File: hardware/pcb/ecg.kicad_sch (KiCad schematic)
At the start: 0 parts

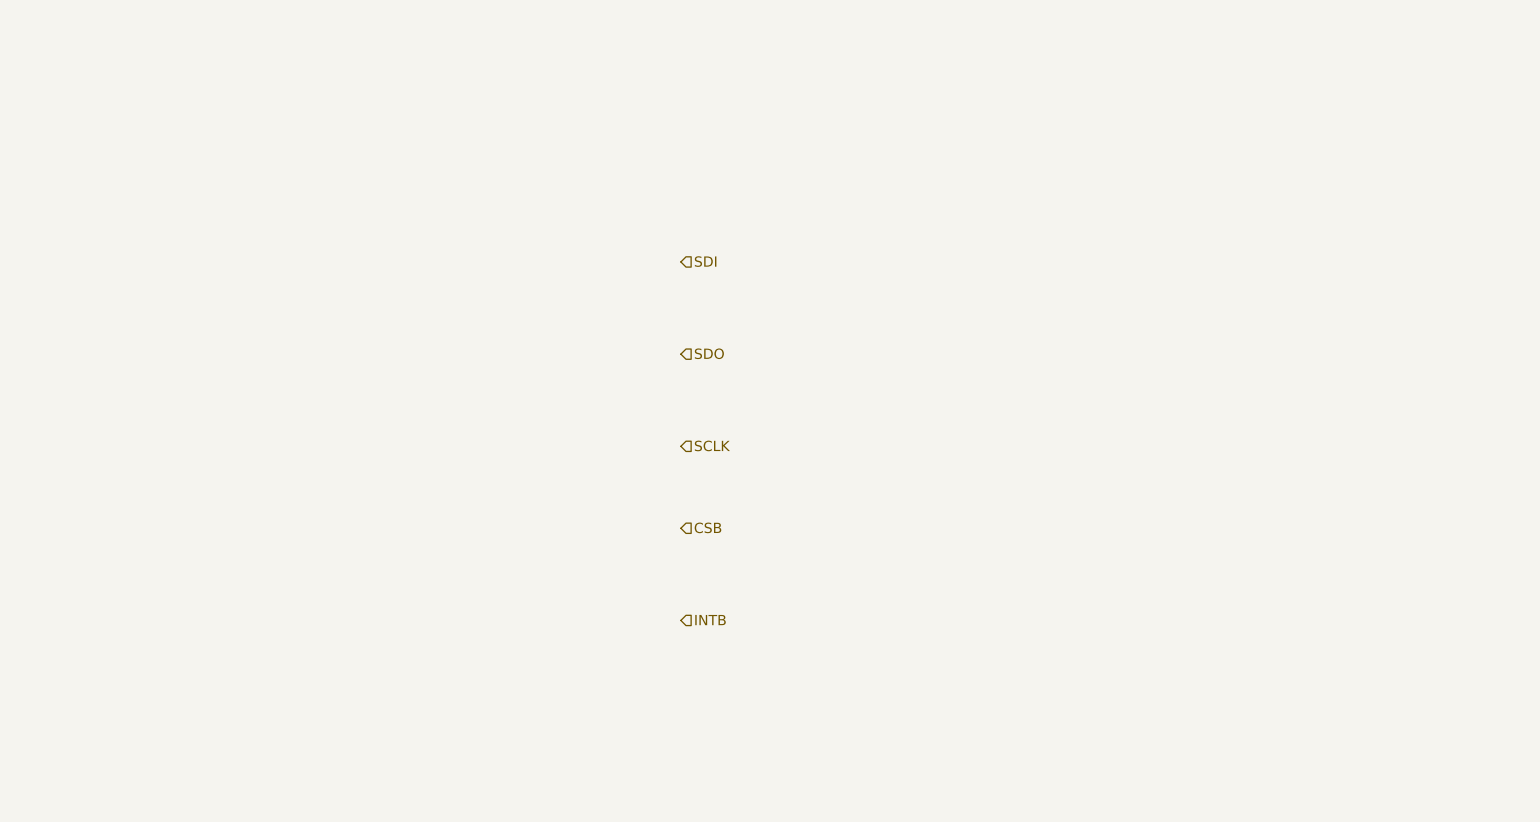
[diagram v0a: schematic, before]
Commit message: Update(hardware): Schematic changes
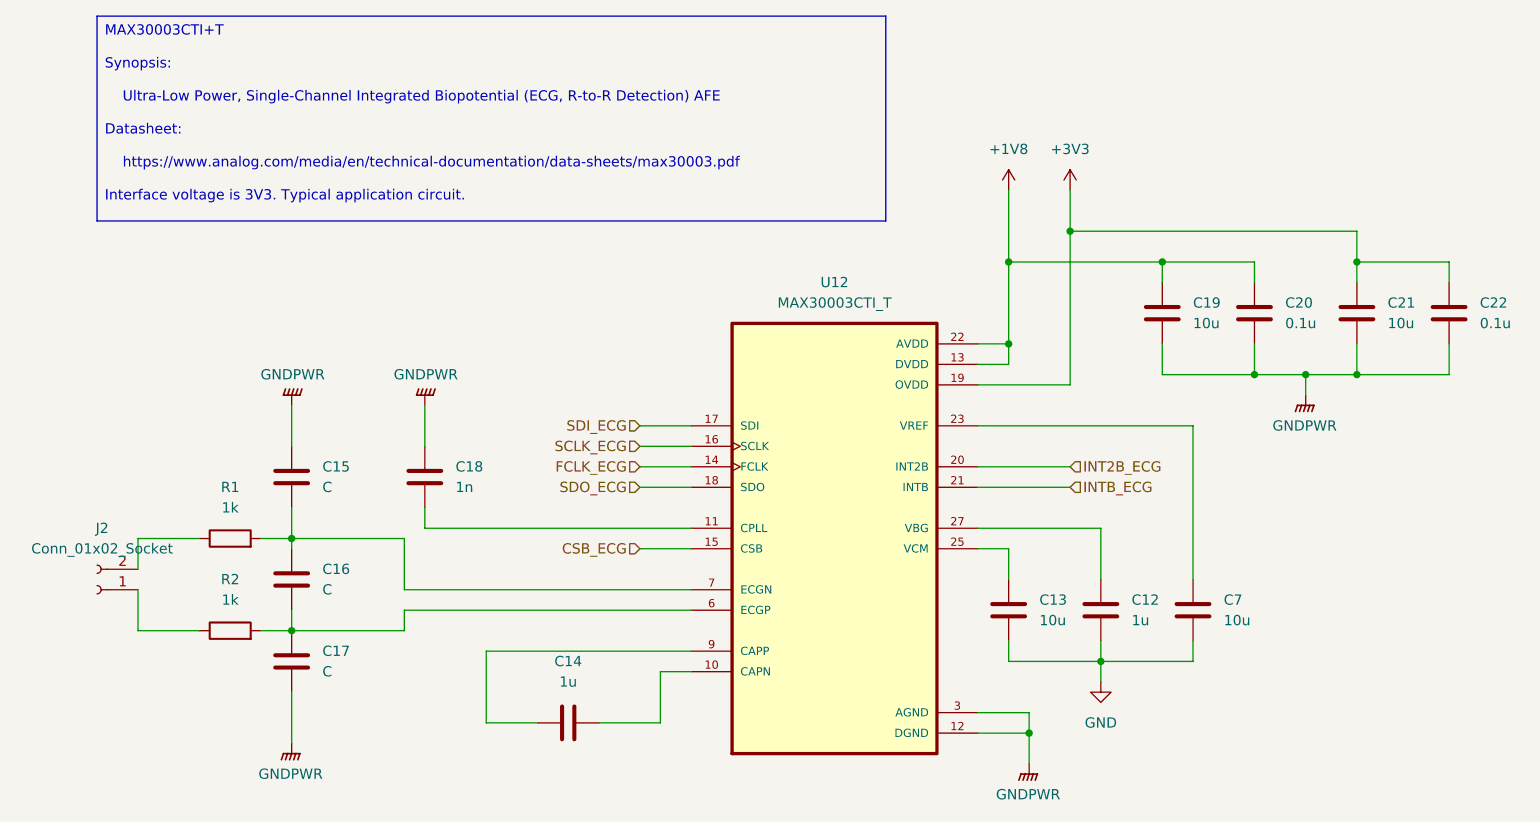
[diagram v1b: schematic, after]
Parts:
- added C12, C14: 1u, footprints:QFN50P500X500X80-29N, symbol Device:C
- added C13, C7: 10u, footprints:QFN50P500X500X80-29N, symbol Device:C
- added C15, C16: C, footprints:QFN50P500X500X80-29N, symbol Device:C
- added C17: C, symbol Device:C
- added C18: 1n, symbol Device:C
- added C19, C21: 10u, symbol Device:C
- added C20, C22: 0.1u, symbol Device:C
- added J2: Conn_01x02_Socket, Connector:Tag-Connect_TC2030-IDC-FP_2x03_P1.27mm_Vertical, symbol Connector:Conn_01x02_Socket
- added R1, R2: 1k, symbol Device:R
- added U12: MAX30003CTI_T, footprints:QFN50P500X500X80-29N, symbol symbols:MAX30003CTI_T
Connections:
- new net: C15.2, C16.1, R1.2, U12.7 (ECGN)
- new net: C16.2, C17.1, R2.2, U12.6 (ECGP)
- new net: J2.1 (Pin_1), R2.1
- new net: J2.2 (Pin_2), R1.1
- new net: C14.1, U12.10 (CAPN)
- new net: C18.2, U12.11 (CPLL)
- new net: C7.2, U12.23 (VREF)
- new net: C13.2, U12.25 (VCM)
- new net: C12.2, U12.27 (VBG)
- new net: C14.2, U12.9 (CAPP)
- new net +1V8: C19.1, C20.1, U12.13 (DVDD), U12.22 (AVDD)
- new net +3V3: C21.1, C22.1, U12.19 (OVDD)
- new net AGND: C15.1, C17.2, C18.1, C19.2, C20.2, C21.2, C22.2, U12.12 (DGND), U12.28 (AGND), U12.29 (AGND), U12.3 (AGND), U12.8 (AGND)
- new net CSB_ECG: U12.15 (CSB)
- new net FCLK_ECG: U12.14 (FCLK)
- new net GND: C12.1, C13.1, C7.1
- new net INT2B_ECG: U12.20 (INT2B)
- new net INTB_ECG: U12.21 (INTB)
- new net SCLK_ECG: U12.16 (SCLK)
- new net SDI_ECG: U12.17 (SDI)
- new net SDO_ECG: U12.18 (SDO)
